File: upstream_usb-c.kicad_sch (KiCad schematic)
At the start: 7 parts

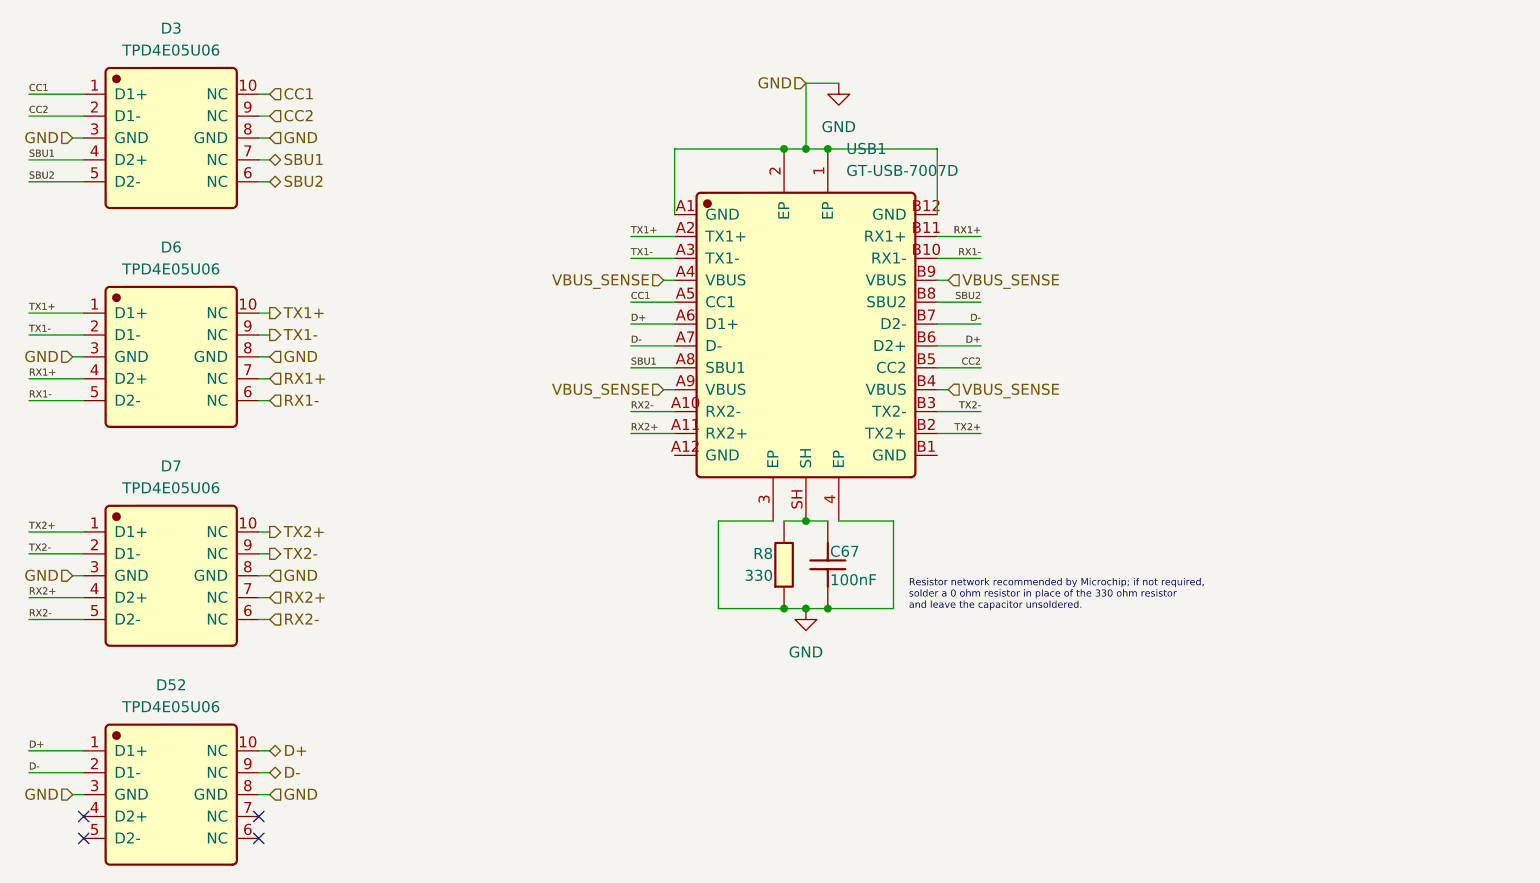
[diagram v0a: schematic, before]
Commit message: Basic Function Review/Documentation of RP2354B
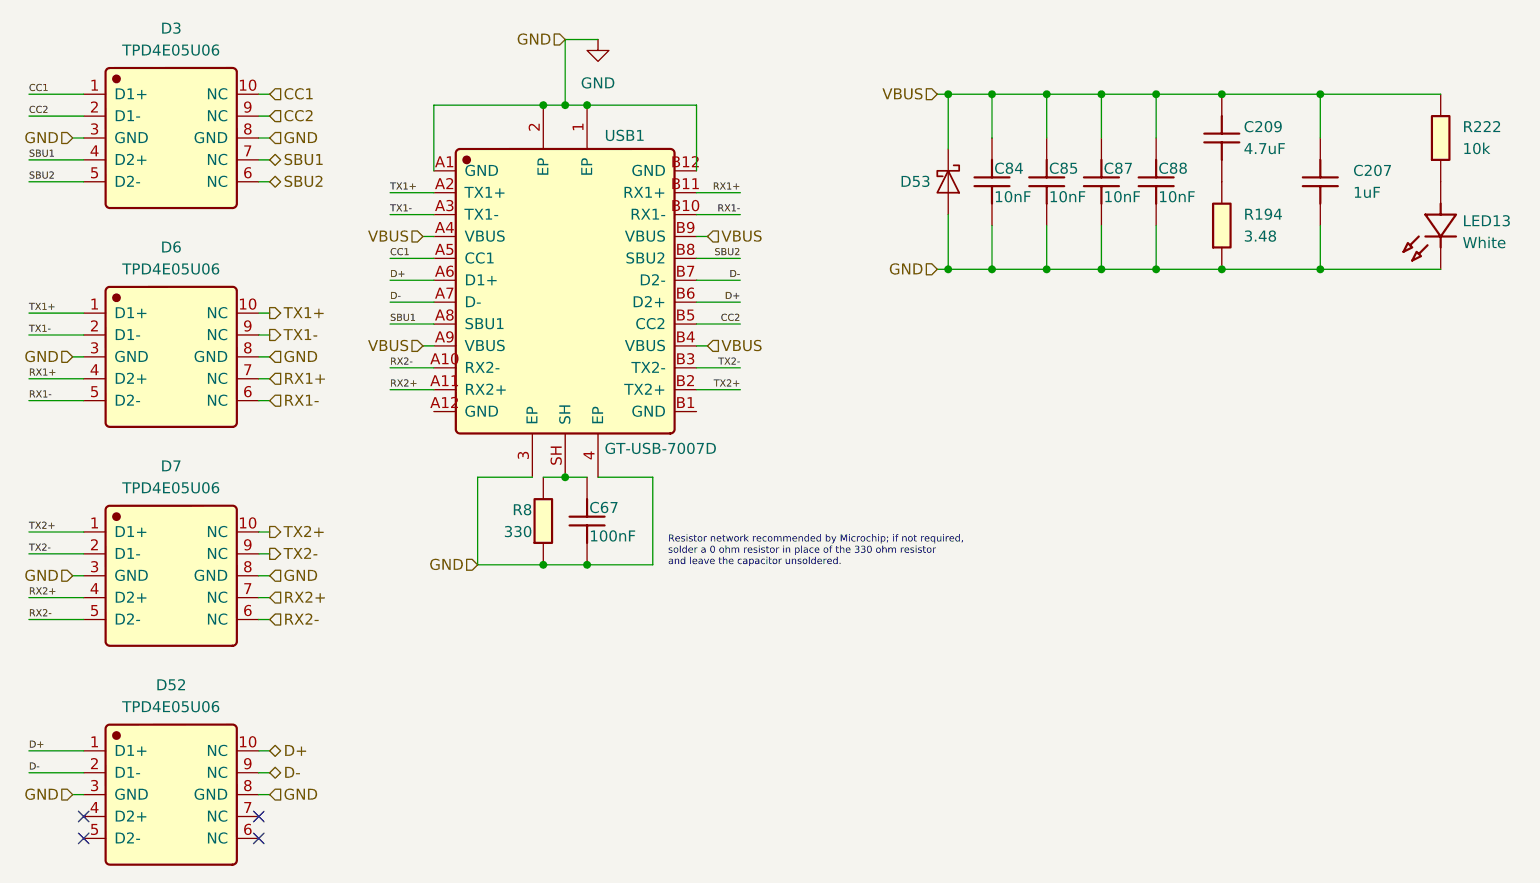
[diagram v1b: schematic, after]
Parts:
- added C207: 1uF, Capacitor_SMD:C_0603_1608Metric, symbol JLCImport:CL10A105KB8NNNC
- added C209: 4.7uF, Capacitor_SMD:C_0603_1608Metric, symbol JLCImport:CL10A475KL8NRNC
- added C84, C85, C87, C88: 10nF, Capacitor_SMD:C_0402_1005Metric, symbol JLCImport:TCC0402X7R103M500AT
- added D53: PMEG3020EH, Diode_SMD:D_SOD-123F, symbol Diode:PMEG3020EH
- added LED13: White, JLCImport:GL0603UW01, symbol JLCImport:GL0603UW01
- added R194: 3.48, Resistor_SMD:R_0603_1608Metric, symbol JLCImport:RS-03L3R48FT
- added R222: 10k, Resistor_SMD:R_0402_1005Metric, symbol JLCImport:0402WGF1002TCE
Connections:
- net GND: now also C207.1, C84.1, C85.1, C87.1, C88.1, D53.2 (A), LED13.2 (C), R194.1
- net VBUS_SENSE renamed VBUS
- net VBUS: now also C207.2, C209.1, C84.2, C85.2, C87.2, C88.2, D53.1 (K), R222.2
- new net: LED13.1 (A), R222.1
- new net: C209.2, R194.2
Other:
- moved on the sheet: C67, R8, USB1
